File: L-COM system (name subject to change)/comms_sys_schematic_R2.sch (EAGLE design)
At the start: 36 parts, among them J1 DCJ0202, Q1 12 Mhz, X3 332-30

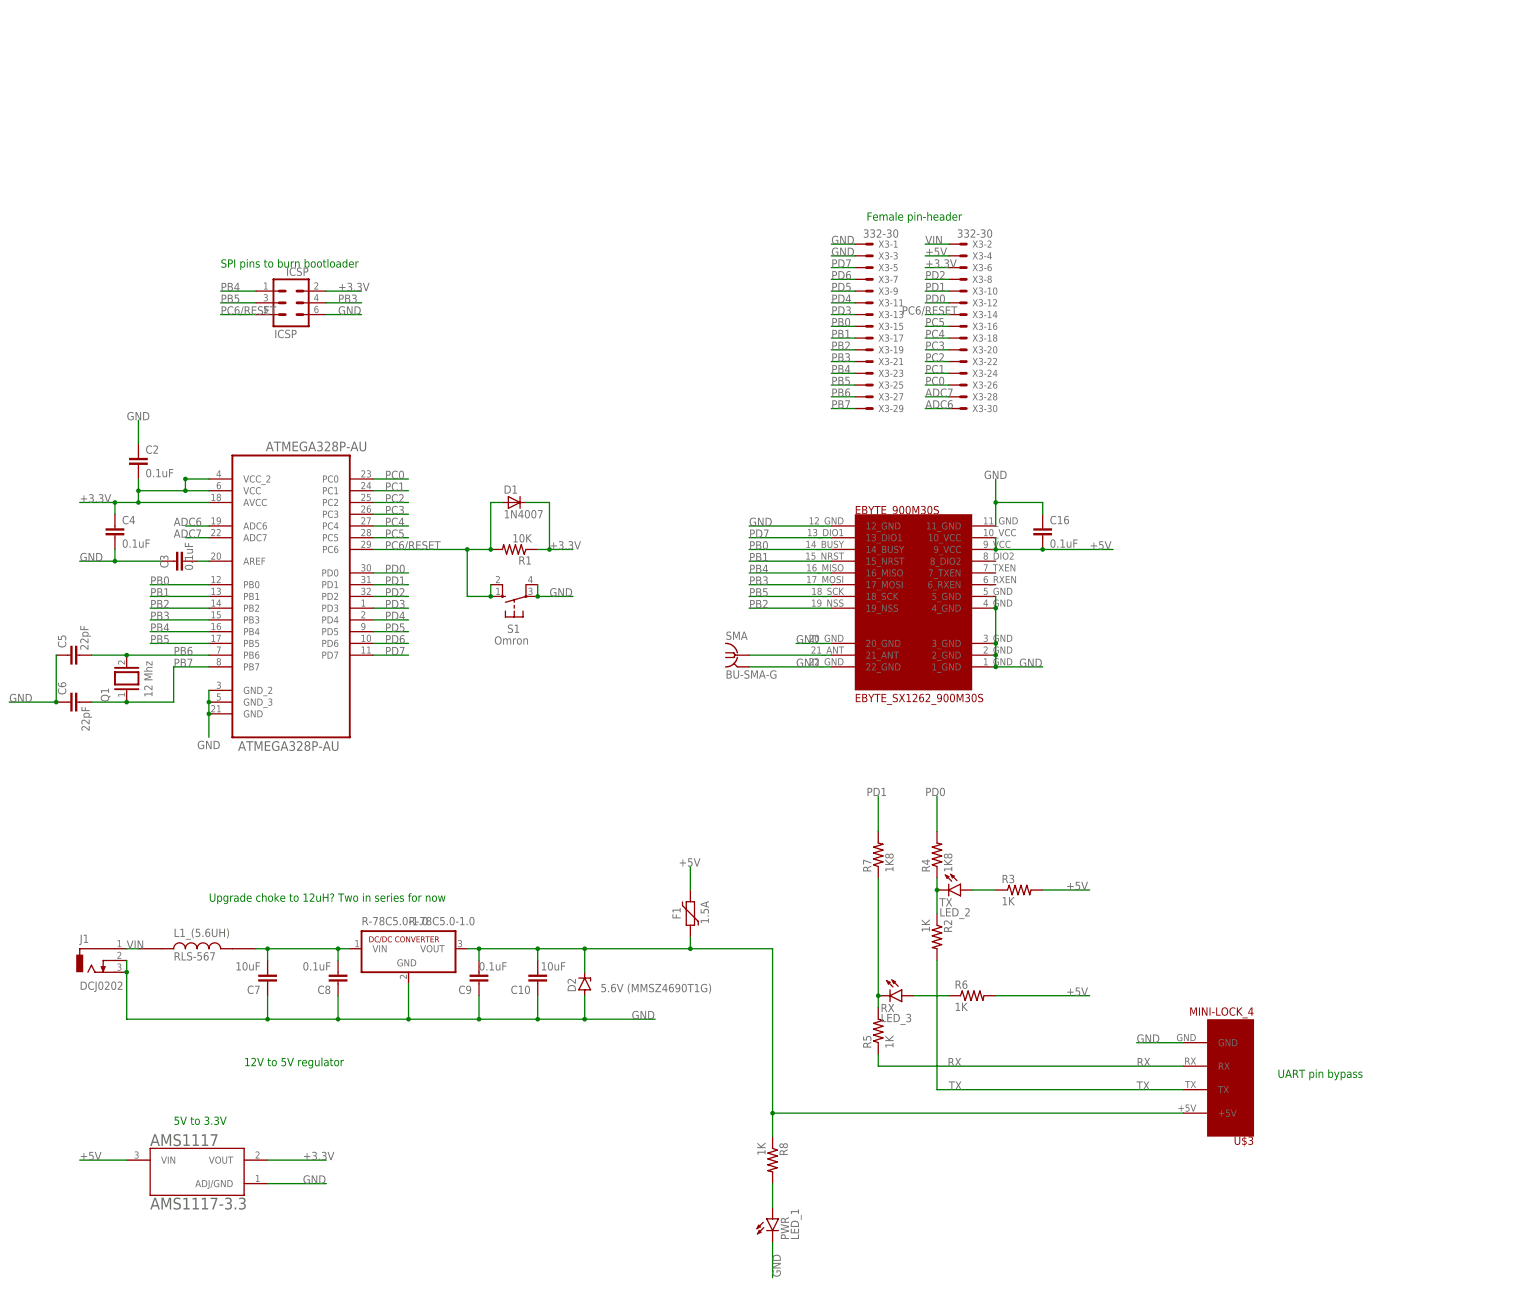
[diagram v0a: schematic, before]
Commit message: Updated board design
Reddit gave some reccomendations
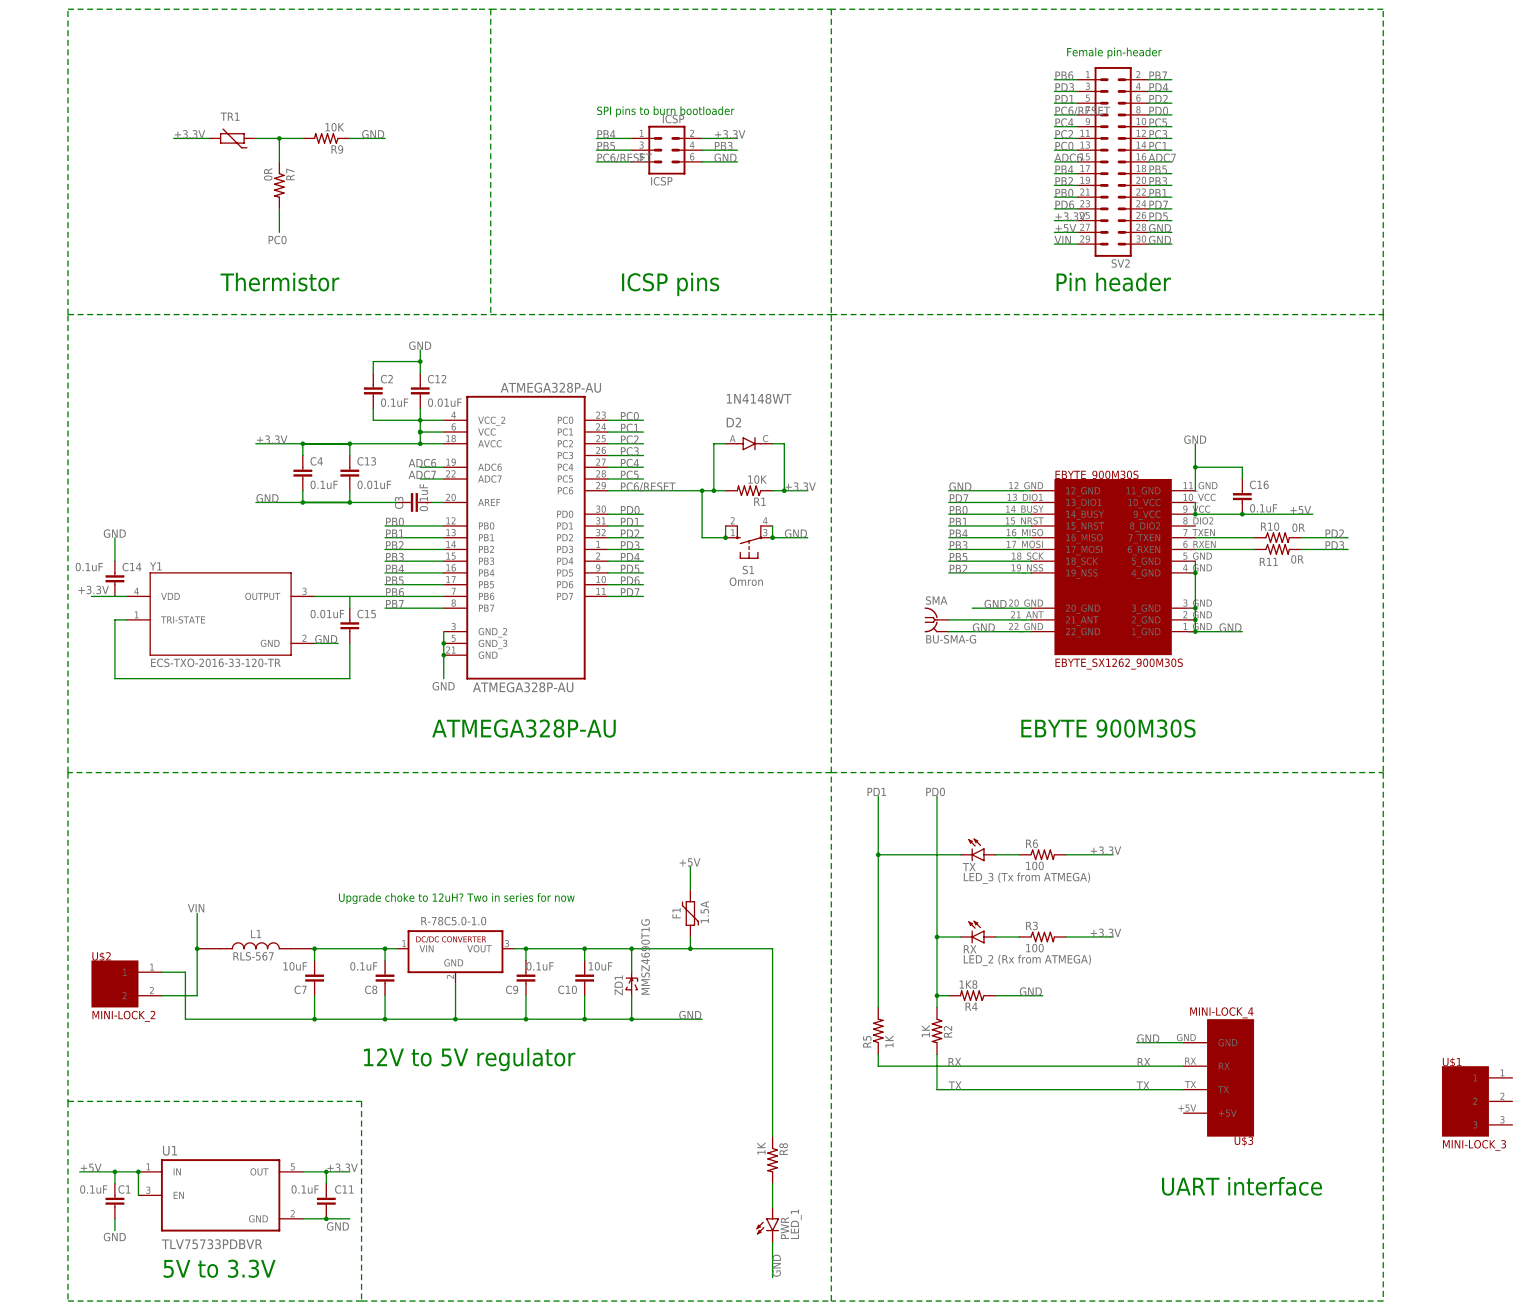
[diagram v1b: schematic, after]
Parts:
- removed AMS1117: AMS1117-3.3, AMS1117-3.3:AMS1117-3.3
- removed C5, C6: 22pF, rcl:C-EUC0805
- removed D1: 1N4007, casovac:1N4007
- removed J1: DCJ0202, con-jack:DCJ0202
- removed L1_(5.6UH): RLS-567, RLS-567:RLS-567
- removed Q1: 12 Mhz, special:XTAL/S
- removed X3: 332-30, con-garry:332-30
- added C1, C11, C14: 0.1uF, rcl:C-EUC0805
- added C12, C13, C15: 0.01uF, rcl:C-EUC0805
- added L1: RLS-567, RLS-567:RLS-567
- added R10, R11: 0R, rcl:R-US_R0805
- added R9: 10K, rcl:R-US_R0805
- added SV2: (no value), con-lstb:MA15-2
- added TR1: (no value), discrete:THERMISTOR_R-2,5
- added U$1: MINI-LOCK_3, cust_parts:MINI-LOCK_3
- added U$2: MINI-LOCK_2, cust_parts:MINI-LOCK_2
- added U1: TLV75733PDBVR, TLV75733PDBVR:TLV75733PDBVR
- added Y1: ECS-TXO-2016-33-120-TR, ECS-TXO-2016-33-120-TR:ECS-TXO-2016-33-120-TR
- added ZD1: MMSZ4690T1G, dp_devices.v6:ZENERSOD-123
- D2: value 5.6V (MMSZ4690T1G) -> 1N4148WT; device diode:ZENER-DIODEDO41Z10 -> 1N4148WT:1N4148WT
- R3, R6: value 1K -> 100
- R7: value 1K8 -> 0R
- RX: value LED_3 -> LED_2 (Rx from ATMEGA)
- TX: value LED_2 -> LED_3 (Tx from ATMEGA)
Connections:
- removed net N$24: R2.1, R4.1, TX.C
- removed net N$25: R5.2, R7.1, RX.C
- new net $N77: R7.1, R9.2, TR1.1
- new net N$5: C15.2, Y1.TRI-STATE
- new net N$6: EBYTE_900M30S.7_TXEN, R10.1
- new net N$7: EBYTE_900M30S.6_RXEN, R11.1
- net +3.3V: now also C11.2, C12.2, C13.1, C14.2, D2.C, R3.2, R6.2, SV2.29, TR1.2, U1.OUT, Y1.VDD; no longer AMS1117.VOUT, D1.C, X3-6.S
- net +5V: now also C1.2, SV2.31, U1.EN, U1.IN; no longer AMS1117.VIN, R3.2, R6.2, X3-4.S
- net ADC6: now also SV2.19; no longer X3-30.S
- net ADC7: now also SV2.20; no longer X3-28.S
- net GND: now also C1.1, C11.1, C12.1, C13.2, C14.1, R4.1, R9.1, SV2.32, SV2.34, U$2.1, U1.GND, Y1.GND, ZD1.A; no longer AMS1117.ADJ/GND, C5.1, C6.1, D2.A, J1.2, J1.3, X3-1.S, X3-3.S
- net N$1: now also ZD1.C; no longer D2.C, U$3.+5V
- net N$12: now also RX.A; no longer TX.A
- net N$16: now also TX.A; no longer RX.A
- net N$27: now also L1.2; no longer L1_(5.6UH).2
- net PB0: now also SV2.25; no longer X3-15.S
- net PB1: now also SV2.26; no longer X3-17.S
- net PB2: now also SV2.23; no longer X3-19.S
- net PB3: now also SV2.24; no longer X3-21.S
- net PB4: now also SV2.21; no longer X3-23.S
- net PB5: now also SV2.22; no longer X3-25.S
- net PB6: now also C15.1, SV2.5, Y1.OUTPUT; no longer C5.2, Q1.2, X3-27.S
- net PB7: now also SV2.6; no longer C6.2, Q1.1, X3-29.S
- net PC0: now also R7.2, SV2.17; no longer X3-26.S
- net PC1: now also SV2.18; no longer X3-24.S
- net PC2: now also SV2.15; no longer X3-22.S
- net PC3: now also SV2.16; no longer X3-20.S
- net PC4: now also SV2.13; no longer X3-18.S
- net PC5: now also SV2.14; no longer X3-16.S
- net PC6/RESET: now also D2.A, SV2.11; no longer D1.A, X3-14.S
- net PD0: now also R2.1, RX.C, SV2.12; no longer X3-12.S
- net PD1: now also R5.2, SV2.9, TX.C; no longer R7.2, X3-10.S
- net PD2: now also R10.2, SV2.10; no longer X3-8.S
- net PD3: now also R11.2, SV2.7; no longer X3-13.S
- net PD4: now also SV2.8; no longer X3-11.S
- net PD5: now also SV2.30; no longer X3-9.S
- net PD6: now also SV2.27; no longer X3-7.S
- net PD7: now also SV2.28; no longer X3-5.S
- net VIN: now also L1.1, SV2.33, U$2.2; no longer J1.1, L1_(5.6UH).1, X3-2.S
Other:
- note added: "ATMEGA328P-AU"
- note added: "EBYTE 900M30S"
- note added: "ICSP pins"
- note added: "Pin header"
- note added: "Thermistor"
- note added: "UART interface"
- note removed: "UART pin bypass"
- moved on the sheet: ATMEGA328P-AU, C10, C16, C2, C3, C4, C7, C8, C9, EBYTE_900M30S, ICSP, R1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
